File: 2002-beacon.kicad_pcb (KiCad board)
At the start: 2 copper layers, 38.1 x 41.3 mm, 16 parts, among them J3 Barrel_Jack, Q1 2N3904, SW1 SW_SPST, U1 L7805, U2 ATtiny85-20PU

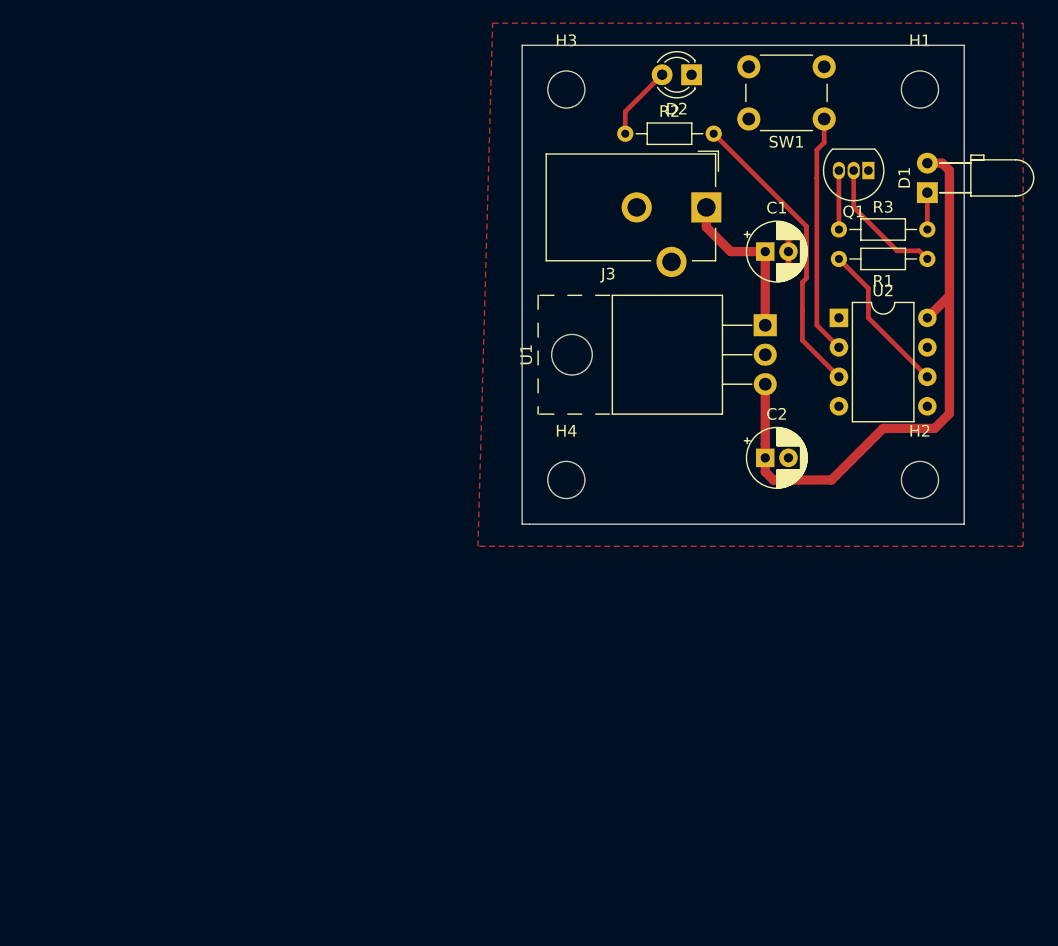
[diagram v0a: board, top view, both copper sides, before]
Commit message: Layout for rev2 done
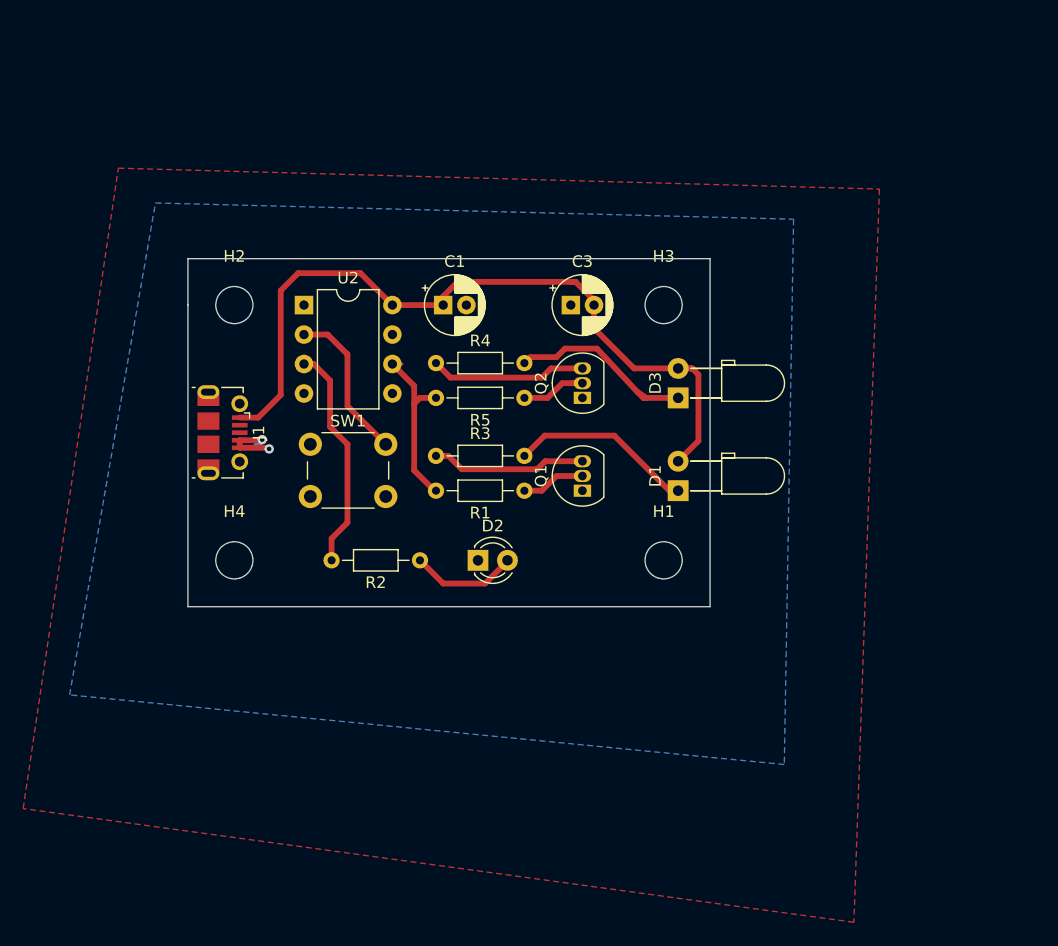
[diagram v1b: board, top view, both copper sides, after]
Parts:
- removed C2: CP1, Capacitor_THT:CP_Radial_D5.0mm_P2.00mm
- removed J3: Barrel_Jack, Connector_BarrelJack:BarrelJack_CUI_PJ-102AH_Horizontal
- removed U1: L7805, Package_TO_SOT_THT:TO-220-3_Horizontal_TabUp
- added C3: C, Capacitor_THT:CP_Radial_D5.0mm_P2.00mm, F.Cu at (95.0, 77.0)
- added D3: LED, LED_THT:LED_D3.0mm_Horizontal_O3.81mm_Z6.0mm, F.Cu at (104.2, 85.0)
- added J1: USB_B, Connector_USB:USB_Micro-B_Molex-105017-0001, F.Cu at (65.0, 88.0)
- added Q2: 2N3904, Package_TO_SOT_THT:TO-92_Inline, F.Cu at (96.0, 85.0)
- added R4: 74, Resistor_THT:R_Axial_DIN0204_L3.6mm_D1.6mm_P7.62mm_Horizontal, F.Cu at (83.4, 82.0)
- added R5: 470, Resistor_THT:R_Axial_DIN0204_L3.6mm_D1.6mm_P7.62mm_Horizontal, F.Cu at (91.0, 85.0)
- C1: value CP1 -> C
- R3: value 90 -> 74
- moved H2 61.0 mm to (66.0, 77.0)
- moved SW1 52.4 mm to (72.5, 89.0), turned to 0 degrees
- moved H1 46.2 mm to (103.0, 99.0)
- moved U2 46.1 mm to (72.0, 77.0)
- moved D2 45.7 mm to (87.0, 99.0), turned to 0 degrees
- moved R2 40.8 mm to (82.0, 99.0), turned to 180 degrees
- moved R1 40.1 mm to (91.0, 93.0)
- moved R3 39.8 mm to (83.4, 90.0)
- moved Q1 37.0 mm to (96.0, 93.0), turned to 90 degrees
- moved D1 33.5 mm to (104.2, 93.0)
- moved H4 29.4 mm to (66.0, 99.0)
- moved C1 28.1 mm to (84.0, 77.0)
- moved H3 20.4 mm to (103.0, 77.0)
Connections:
- C1 pad 1: Net-(C1-Pad1) -> +5V
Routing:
- net +5V: track 51.9 -> 76.4 mm
- net Net-(D3-Pad1): track 0.00 -> 16.5 mm
- net Net-(C1-Pad1): track 14.0 -> 0.00 mm
- net Net-(Q2-Pad3): track 0.00 -> 13.5 mm
- net Net-(D1-Pad1): track 3.17 -> 15.9 mm
- net Net-(R1-Pad2): track 13.3 -> 23.3 mm
- net Net-(Q1-Pad3): track 5.08 -> 13.4 mm
- net Net-(SW1-Pad1): track 20.7 -> 13.6 mm
- net Net-(R2-Pad2): track 25.7 -> 19.5 mm
- net Net-(Q1-Pad2): track 11.4 -> 5.53 mm
- net Net-(Q2-Pad2): track 0.00 -> 5.53 mm
- net Net-(D2-Pad2): track 6.40 -> 9.24 mm
- net GND: track 3.60 -> 6.04 mm, vias 0 -> 2
- added copper zone on F.Cu, net +5V
- added copper zone on B.Cu, net GND
- removed copper zone on F.Cu, net GND
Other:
- board size 38.1 x 41.3 mm -> 45 x 30 mm
